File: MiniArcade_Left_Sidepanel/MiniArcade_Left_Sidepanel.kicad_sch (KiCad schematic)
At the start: 6 parts, among them J1 M20-7910242R, J2 M20-7910542R, J3 M20-7910642R, J4 USB_C_PWR_Connector

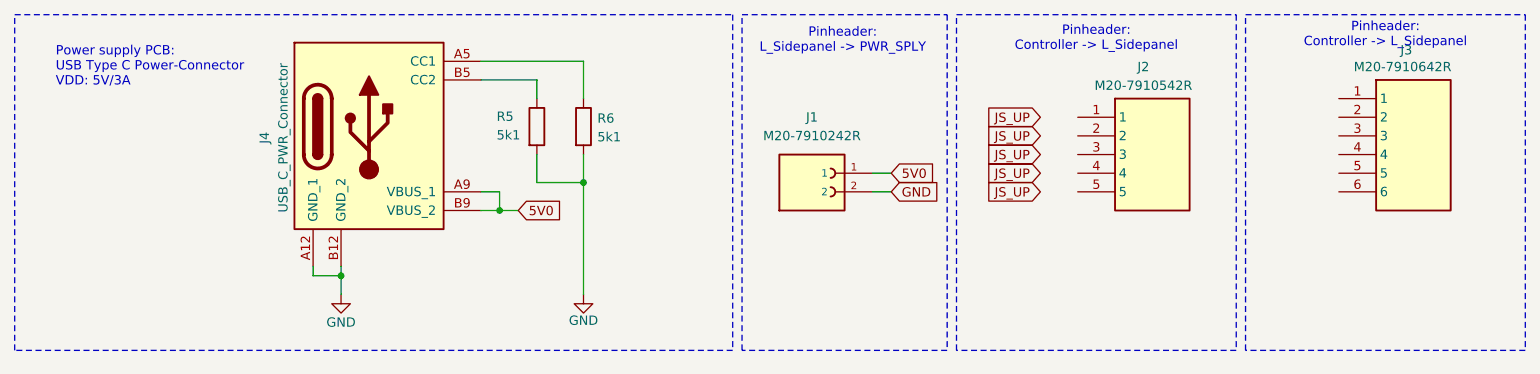
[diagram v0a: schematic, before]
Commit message: 17 11 2025
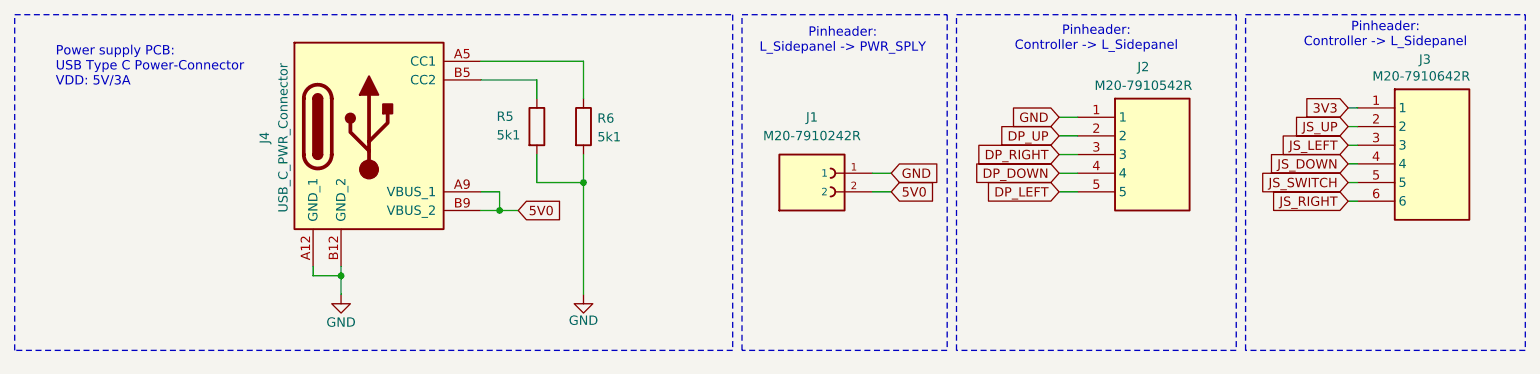
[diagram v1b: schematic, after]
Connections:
- net 5V0: now also J1.2; no longer J1.1
- net GND: now also J1.1, J2.1; no longer J1.2
- net JS_UP: now also J3.2
- net DP_UP: now reaches J2.2
- net DP_RIGHT: now reaches J2.3
- net DP_DOWN: now reaches J2.4
- net DP_LEFT: now reaches J2.5
- net 3V3: now reaches J3.1
- net JS_LEFT: now reaches J3.3
- net JS_DOWN: now reaches J3.4
- net JS_SWITCH: now reaches J3.5
- net JS_RIGHT: now reaches J3.6
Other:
- moved on the sheet: J3

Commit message: 19 11 2025
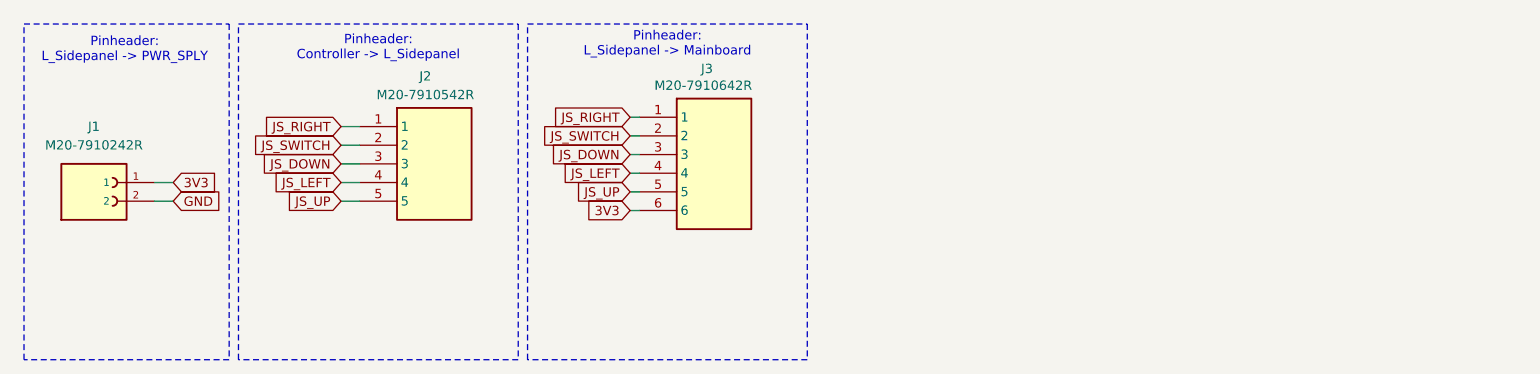
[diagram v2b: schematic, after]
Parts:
- removed J4: USB_C_PWR_Connector, MiniArcadeLeftSidepanel:USB4125GFA, symbol MiniArcadePwrSupply:USB_C_PWR_CONNECTOR
- removed R5, R6: 5k1, Resistor_SMD:R_0603_1608Metric_Pad0.98x0.95mm_HandSolder, symbol Device:R
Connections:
- net 5V0 is gone; now on net GND: J1.2
- net DP_DOWN is gone; now on net JS_LEFT: J2.4
- net DP_LEFT is gone; now on net JS_UP: J2.5
- net DP_RIGHT is gone; now on net JS_DOWN: J2.3
- net DP_UP is gone; now on net JS_SWITCH: J2.2
- net 3V3: now also J1.1, J3.6; no longer J3.1
- net GND: no longer J1.1, J2.1
- net JS_DOWN: now also J3.3; no longer J3.4
- net JS_LEFT: now also J3.4; no longer J3.3
- net JS_RIGHT: now also J2.1, J3.1; no longer J3.6
- net JS_SWITCH: now also J3.2; no longer J3.5
- net JS_UP: now also J3.5; no longer J3.2
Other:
- note added: "Pinheader: L_Sidepanel -> Mainboard"
- note removed: "Power supply PCB: USB Type C Power-Connector VDD: 5V/3A"
- moved on the sheet: J1, J2, J3
